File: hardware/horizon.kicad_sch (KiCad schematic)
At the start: 39 parts, among them J1 Conn_01x02_Pin, J2 Conn_01x06_Pin, J3 USB_C_Receptacle_USB2.0_14P, J4 Conn_01x14_Pin, J5 Conn_01x02_Socket, J6 Conn_01x02_Pin, Q1 NPN, SW1 SW_Push, SW2 SW_Push, U1 ESP32-S3, U2 NCP1529A, U3 W25Q128JVS, U4 BQ24074RGT, U5 DRV2605LDGS, Y1 CDX-1293

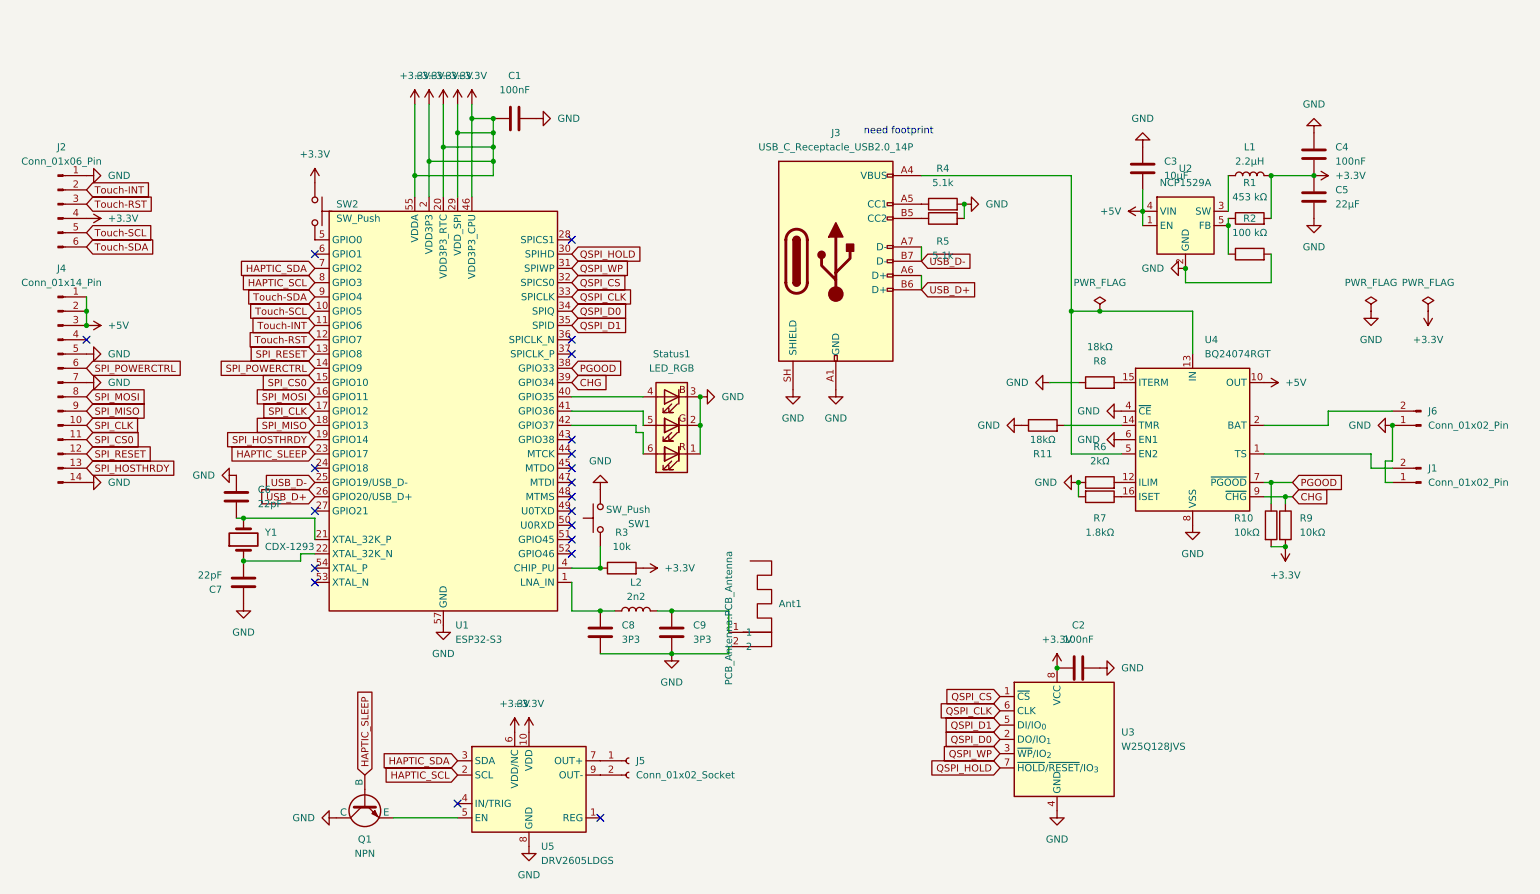
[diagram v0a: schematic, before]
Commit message: Redoing pcb and fixed schem
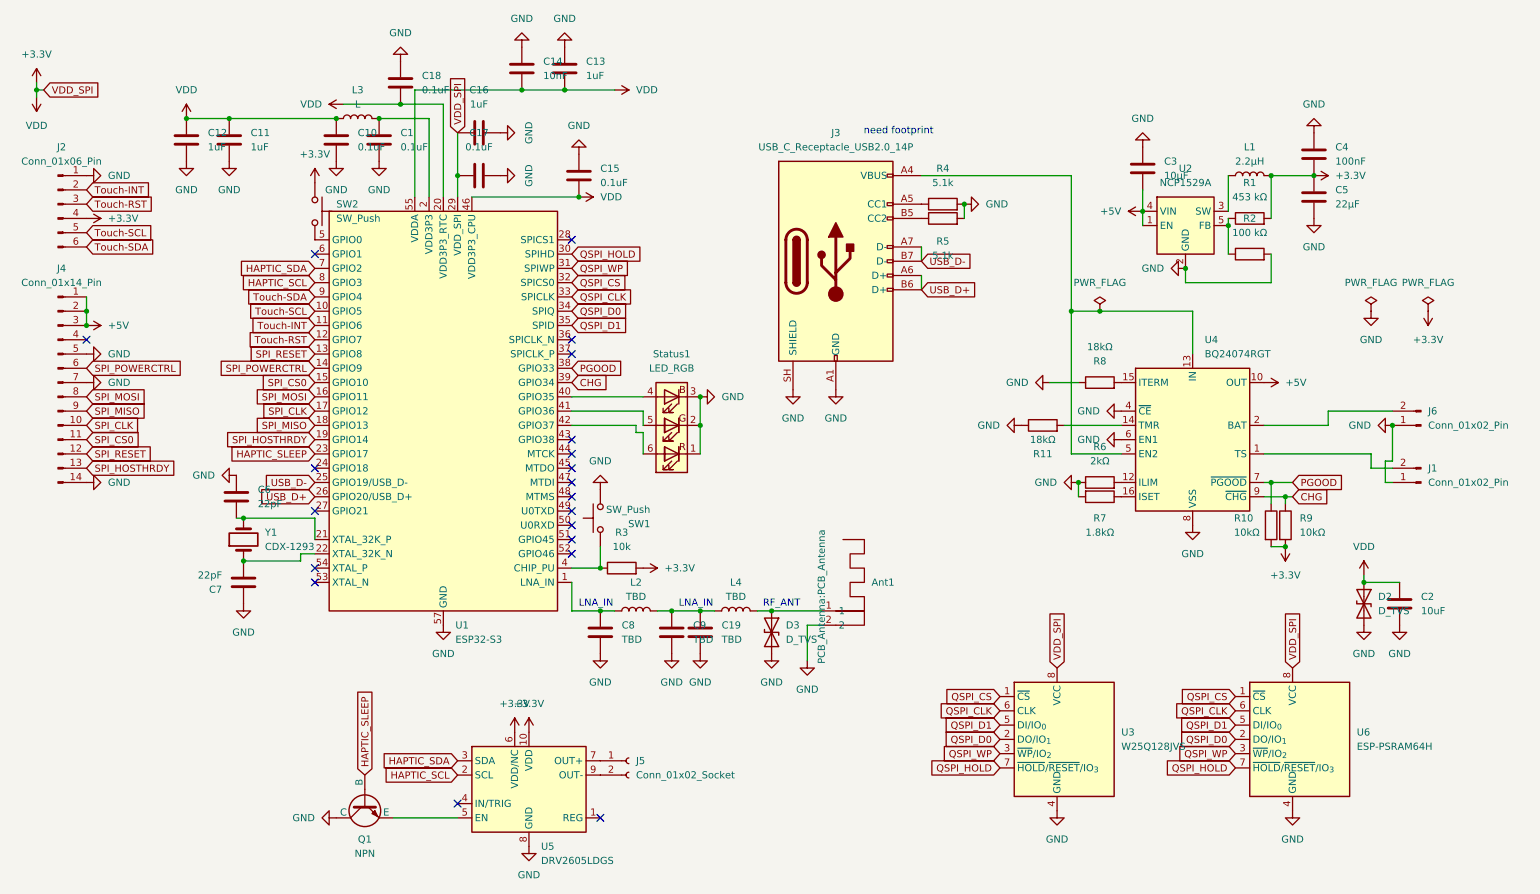
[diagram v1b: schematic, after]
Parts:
- added C10, C15, C17, C18: 0.1uF, Capacitor_SMD:C_0201_0603Metric, symbol Device:C
- added C11, C12, C13, C16: 1uF, Capacitor_SMD:C_0201_0603Metric, symbol Device:C
- added C14: 10nF, Capacitor_SMD:C_0201_0603Metric, symbol Device:C
- added C19: TBD, Capacitor_SMD:C_0201_0603Metric, symbol Device:C
- added D2, D3: D_TVS, Diode_SMD:D_0402_1005Metric, symbol Device:D_TVS
- added L3: L, Inductor_SMD:L_Bourns_SDR0604, symbol Device:L
- added L4: TBD, Inductor_SMD:L_Bourns_SDR0604, symbol Device:L
- added U6: ESP-PSRAM64H, Package_SO:SOIC-8_5.3x5.3mm_P1.27mm, symbol Memory_Flash:W25Q128JVS
- C1: value 100nF -> 0.1uF; footprint Capacitor_SMD:C_0201_0603Metric -> Diode_SMD:D_0402_1005Metric
- C2: value 100nF -> 10uF
- C8, C9: value 3P3 -> TBD
- L2: value 2n2 -> TBD
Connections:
- net +3.3V: now also C10.1, C11.1, C12.1, C13.1, C14.1, C15.1, C16.1, C17.1, C18.1, D2.1 (A1), L3.1, U6.8 (VCC); no longer C1.1, U1.2 (VDD3P3), U1.3 (VDD3P3)
- net GND: now also C10.2, C11.2, C12.2, C13.2, C14.2, C15.2, C16.2, C17.2, C18.2, C19.2, D2.2 (A2), D3.2 (A2), U6.4 (GND)
- net QSPI_CLK: now also U6.6 (CLK)
- net QSPI_CS: now also U6.1 (~{CS})
- net QSPI_D0: now also U6.2 (DO/IO_{1})
- net QSPI_D1: now also U6.5 (DI/IO_{0})
- net QSPI_HOLD: now also U6.7 (~{HOLD}/~{RESET}/IO_{3})
- net QSPI_WP: now also U6.3 (~{WP}/IO_{2})
- net at C9.1, L2.2: now also C19.1, L4.1; no longer Ant1.1
- new net: C1.1, L3.2, U1.2 (VDD3P3), U1.3 (VDD3P3)
- new net: Ant1.1, D3.1 (A1), L4.2
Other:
- note added: "LNA_IN"
- note added: "RF_ANT"
